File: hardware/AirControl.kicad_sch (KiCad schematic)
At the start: 8 parts, among them Q13 2SK3065, Q4 2SK3065, Q5 2SK3065

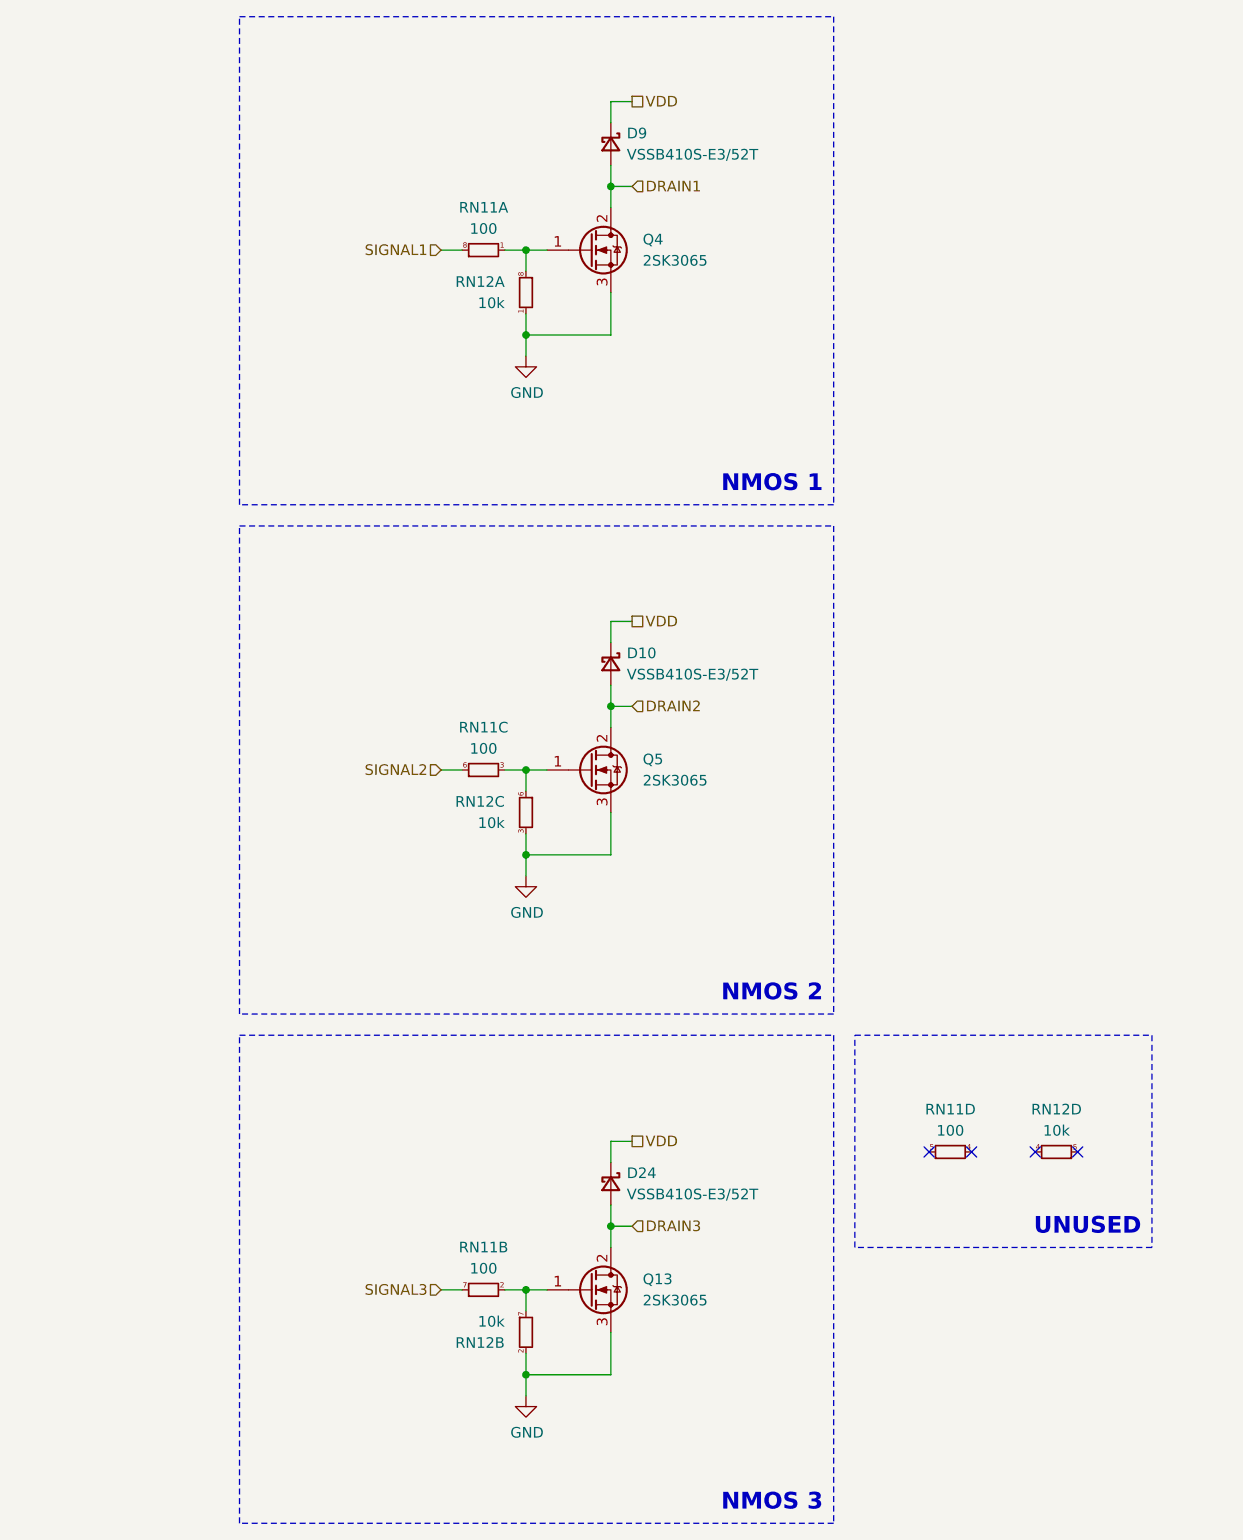
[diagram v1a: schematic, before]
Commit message: schematic done
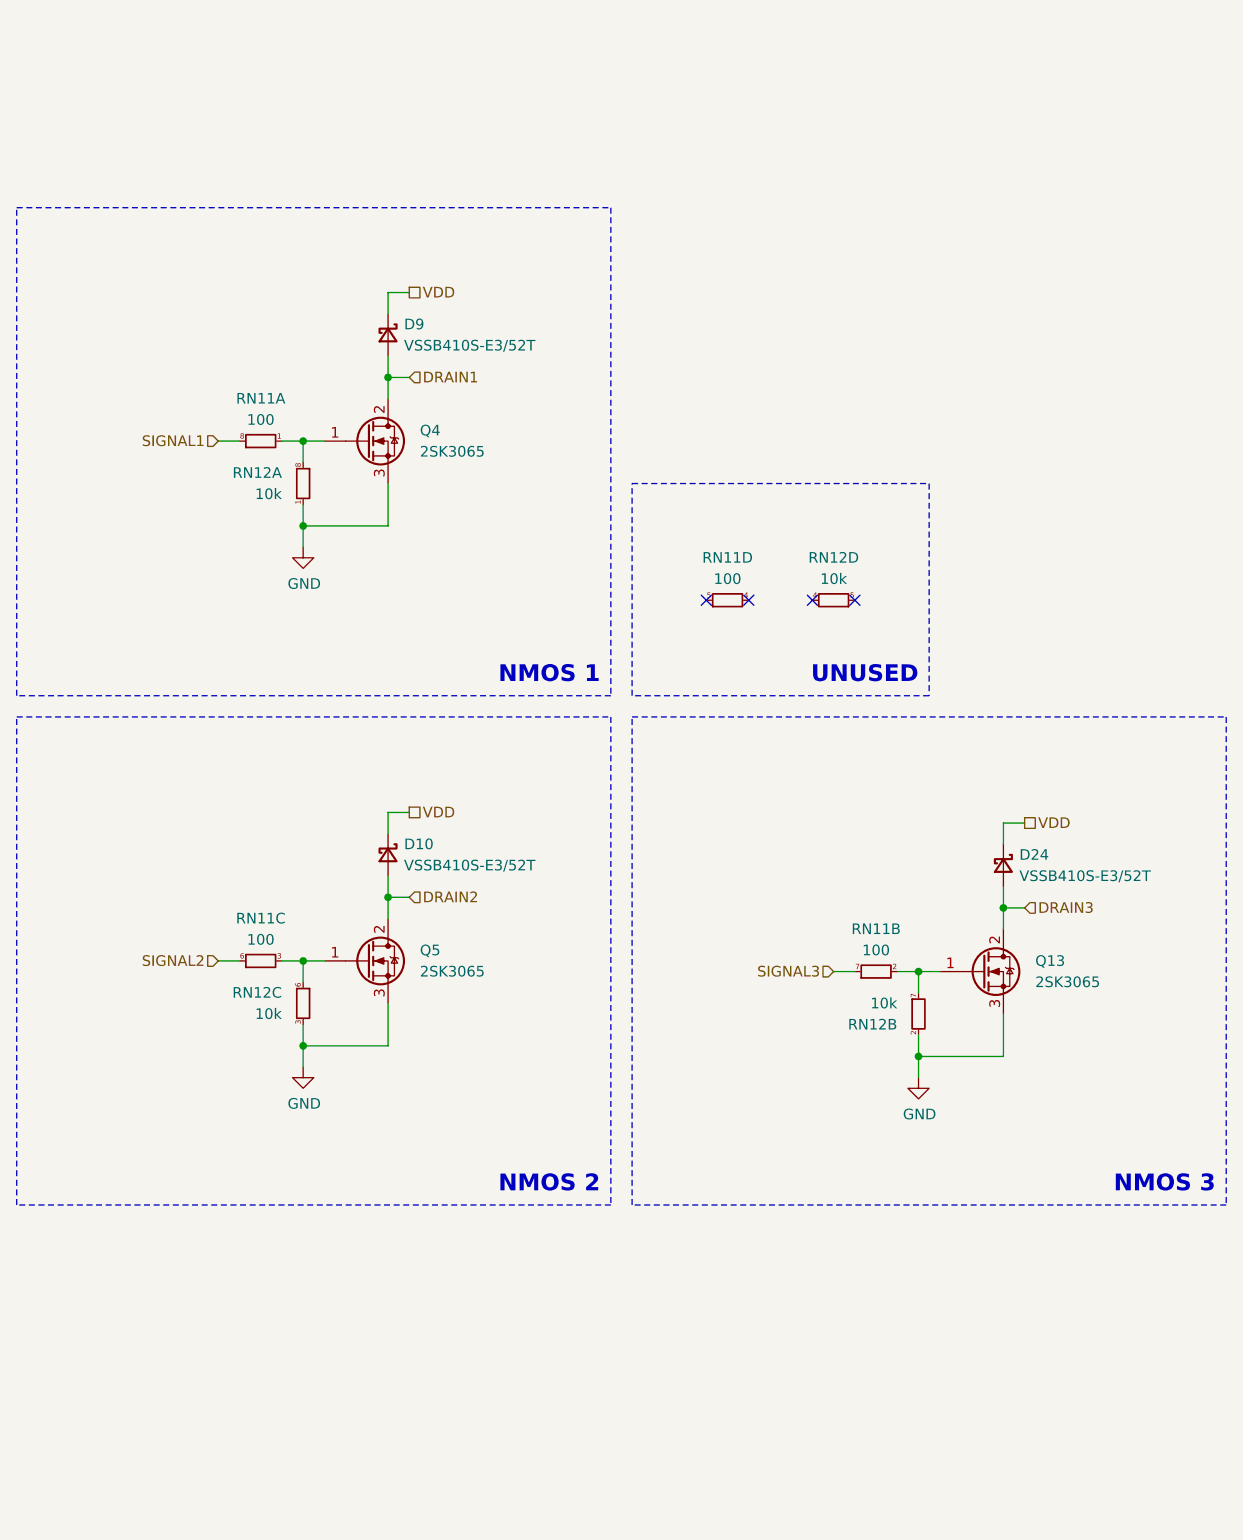
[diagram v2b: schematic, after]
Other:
- moved on the sheet: D10, D24, D9, Q13, Q4, Q5, RN11A, RN11B, RN11C, RN11D, RN12A, RN12B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
